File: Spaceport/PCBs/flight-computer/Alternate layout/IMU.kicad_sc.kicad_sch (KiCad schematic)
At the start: 3 parts, among them U2 BMI088

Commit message: silkscreen changes + minor layout changes
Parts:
- U2: footprint BMI088:PQFN50P450X300X100-16N -> Package_LGA:Bosch_LGA-16_4.5x3mm_P0.5mm_LayoutBorder7x1y_ClockwisePinNumbering
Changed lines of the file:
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@@
 			)
 		)
-		(property "Footprint" "BMI088:PQFN50P450X300X100-16N"
+		(property "Footprint" "Package_LGA:Bosch_LGA-16_4.5x3mm_P0.5mm_LayoutBorder7x1y_ClockwisePinNumbering"
 			(at 152.4 100.33 0)
 			(effects

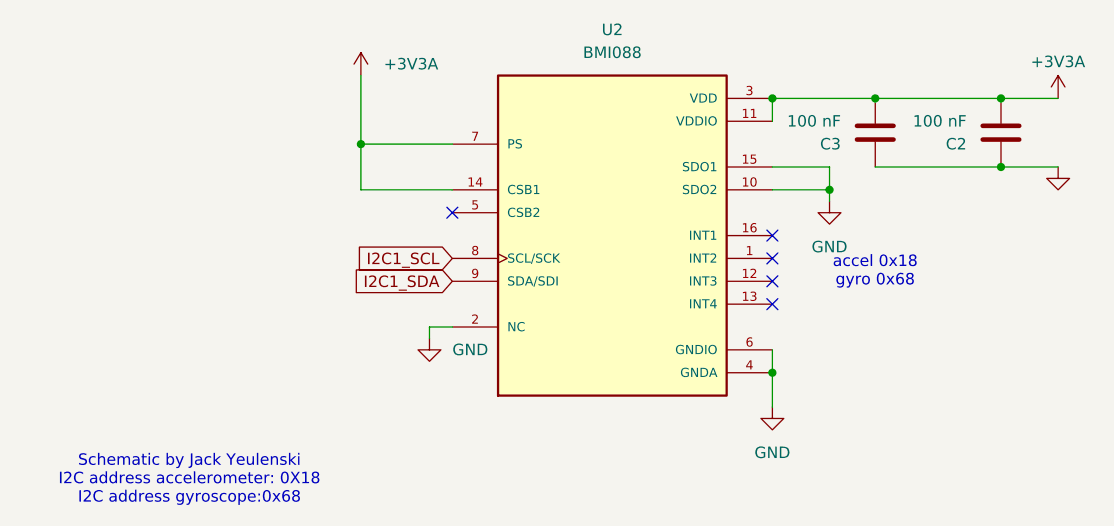
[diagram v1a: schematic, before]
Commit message: removed all global labels
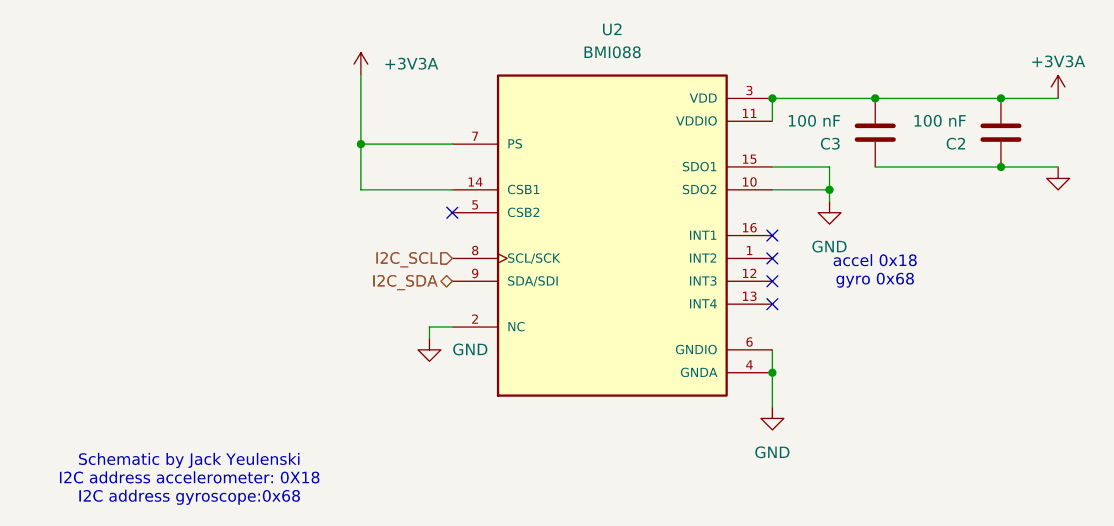
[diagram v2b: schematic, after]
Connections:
- net I2C1_SCL renamed I2C_SCL
- net I2C1_SDA renamed I2C_SDA
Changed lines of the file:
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@@
 		)
 	)
-	(global_label "I2C1_SCL"
+	(hierarchical_label "I2C_SCL"
 		(shape input)
 		(at 134.62 102.87 180)
-		(fields_autoplaced yes)
 		(effects
 			(font
@@
 			(justify right)
 		)
-		(property "Intersheetrefs" "${INTERSHEET_REFS}"
-			(at 122.8658 102.87 0)
-			(effects
-				(font
-					(size 1.27 1.27)
-				)
-				(justify right)
-				(hide yes)
-			)
-		)
 	)
-	(global_label "I2C1_SDA"
-		(shape input)
+	(hierarchical_label "I2C_SDA"
+		(shape bidirectional)
 		(at 134.62 105.41 180)
-		(fields_autoplaced yes)
 		(effects
 			(font
@@
 			(justify right)
 		)
-		(property "Intersheetrefs" "${INTERSHEET_REFS}"
-			(at 122.8053 105.41 0)
-			(effects
-				(font
-					(size 1.27 1.27)
-				)
-				(justify right)
-				(hide yes)
-			)
-		)
 	)
